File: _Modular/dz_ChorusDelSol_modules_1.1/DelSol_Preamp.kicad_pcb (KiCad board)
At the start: 2 copper layers, 110.5 x 38.1 mm, 79 parts, among them J1 Filter Switch, J2 BBD Drive, J3 Dry LMR In, J4 Eq Pot Hi, J5 Eq Pot Mid, J6 Eq Pot Low, J7 Power, U1 LM2904, U2 MCP601, U3 LM2902

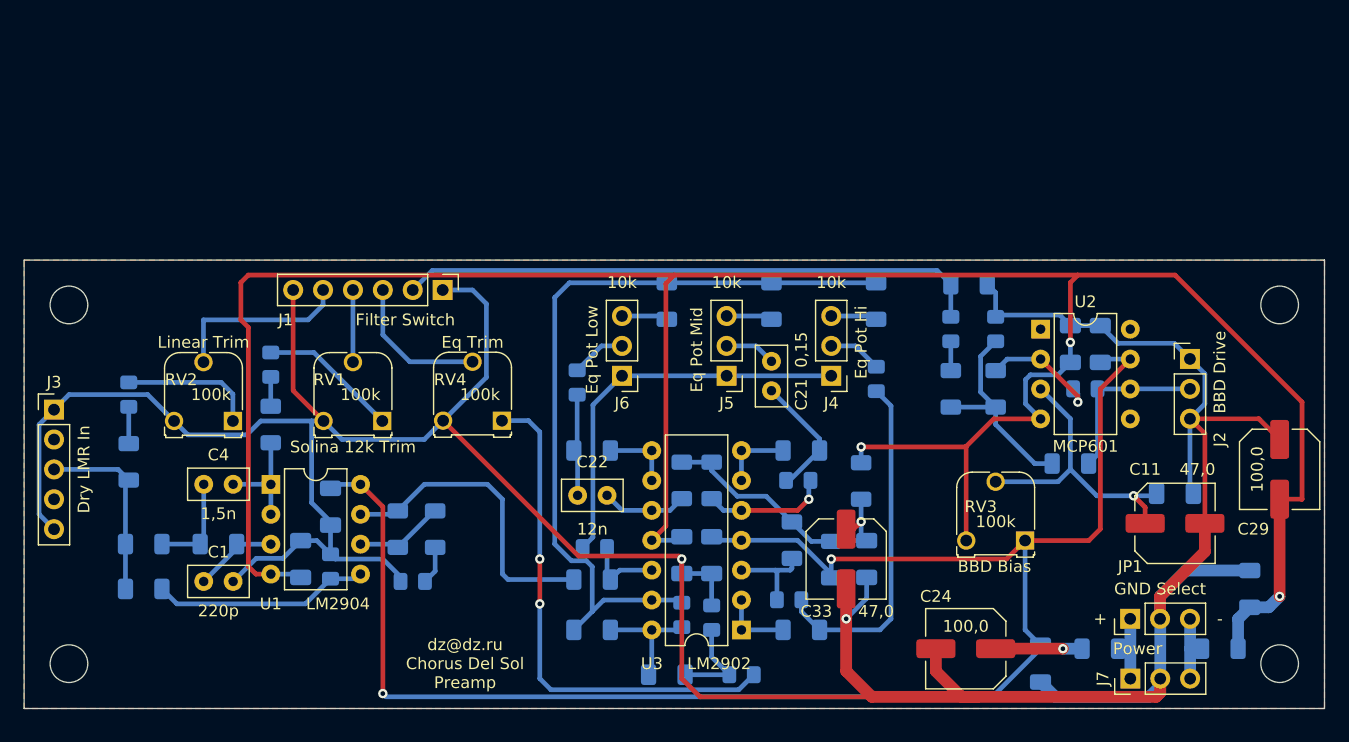
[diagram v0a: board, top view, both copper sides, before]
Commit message: up
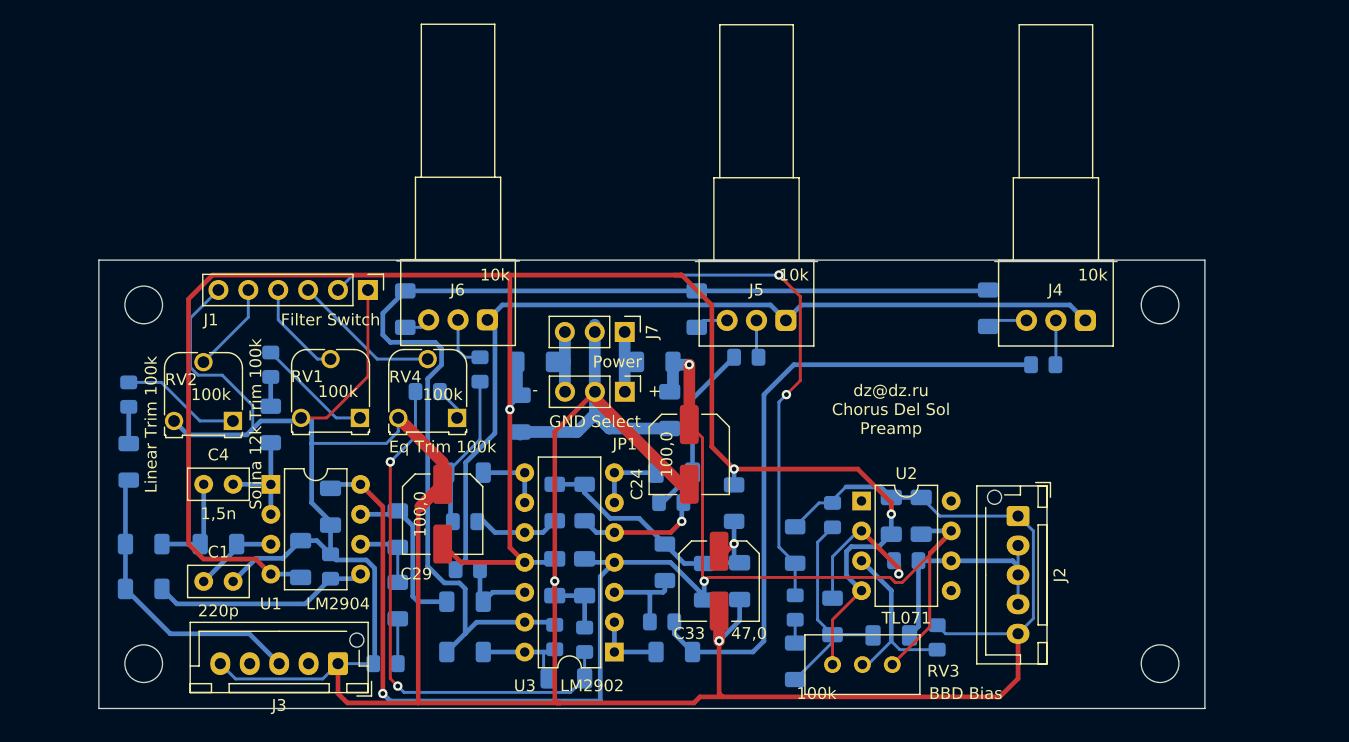
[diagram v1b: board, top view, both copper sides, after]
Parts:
- removed C12: 0,1, Capacitor_SMD:C_1206_3216Metric_Pad1.33x1.80mm_HandSolder
- C11: value 47,0 -> 10,0; footprint Capacitor_SMD:C_Elec_6.3x5.8 -> Capacitor_SMD:C_0805_2012Metric_Pad1.18x1.45mm_HandSolder; moved to B.Cu
- C21, C22: footprint Capacitor_THT:C_Disc_D5.0mm_W2.5mm_P2.50mm -> Capacitor_SMD:C_0805_2012Metric_Pad1.18x1.45mm_HandSolder; moved to B.Cu
- J2: footprint Connector_PinHeader_2.54mm:PinHeader_1x03_P2.54mm_Vertical -> Connector_JST:JST_XH_B5B-XH-AM_1x05_P2.50mm_Vertical
- J3: footprint Connector_PinHeader_2.54mm:PinHeader_1x05_P2.54mm_Vertical -> Connector_JST:JST_XH_B5B-XH-AM_1x05_P2.50mm_Vertical
- J4: value Eq Pot Hi -> Eq Pot 10k; footprint Connector_PinHeader_2.54mm:PinHeader_1x03_P2.54mm_Vertical -> Potentiometer_THT:Potentiometer_Alps_RK097_Single_Horizontal
- J5: value Eq Pot Mid -> Eq Pot 10k; footprint Connector_PinHeader_2.54mm:PinHeader_1x03_P2.54mm_Vertical -> Potentiometer_THT:Potentiometer_Alps_RK097_Single_Horizontal
- J6: value Eq Pot Low -> Eq Pot 10k; footprint Connector_PinHeader_2.54mm:PinHeader_1x03_P2.54mm_Vertical -> Potentiometer_THT:Potentiometer_Alps_RK097_Single_Horizontal
- RV1: value Solina 12k Trim -> Solina 12k Trim 100k
- RV2: value Linear Trim -> Linear Trim 100k
- RV3: footprint Potentiometer_THT:Potentiometer_Runtron_RM-065_Vertical -> Potentiometer_THT:Potentiometer_Bourns_3296W_Vertical
- RV4: value Eq Trim -> Eq Trim 100k
- U2: value MCP601 -> TL071
- moved C29 71.2 mm to (87.6, 39.4)
- moved C30 63.8 mm to (94.2, 30.8), turned to 90 degrees
- moved R26 63.1 mm to (95.5, 26.4), turned to 180 degrees
- moved J7 52.1 mm to (103.1, 23.9), turned to -90 degrees
- moved JP1 47.1 mm to (103.1, 29.0), turned to -90 degrees
- moved R24 45.0 mm to (105.7, 26.4), turned to 0 degrees
- moved C25 38.2 mm to (106.9, 30.5)
- moved C13 35.9 mm to (86.4, 28.9)
- moved J3 32.4 mm to (78.7, 52.1), turned to 180 degrees
- moved C24 28.7 mm to (108.6, 34.3), turned to -90 degrees
- moved C7 27.1 mm to (117.6, 47.3)
- moved R6 26.7 mm to (117.6, 51.9)
- moved R8 26.6 mm to (117.6, 42.0), turned to -90 degrees
- moved R7 23.8 mm to (120.8, 48.1)
- moved C11 22.4 mm to (129.7, 49.8), turned to 90 degrees
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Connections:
- J2 pad 3: GND -> Net-(C6-Pad1)
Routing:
- net /-V: track 216.9 -> 166.7 mm
- net Net-(C14-Pad1): track 33.8 -> 75.9 mm
- net Net-(C13-Pad1): track 43.7 -> 2.85 mm, vias 2 -> 0
- net Net-(C13-Pad2): track 8.19 -> 45.0 mm, vias 0 -> 2
- net Net-(C17-Pad1): track 66.9 -> 96.6 mm
- net /+V: track 153.5 -> 128.0 mm
- net Net-(C18-Pad2): track 29.5 -> 54.3 mm
- net Net-(C7-Pad1): track 49.7 -> 66.4 mm, vias 0 -> 2
- net GND: track 298.8 -> 312.3 mm
- net Net-(R10-Pad1): track 26.3 -> 14.2 mm
- net Net-(RV3-Pad2): track 25.9 -> 15.4 mm, vias 1 -> 0
- net /Dry Mix: track 16.1 -> 25.1 mm
- net Net-(J1-Pad5): track 15.5 -> 7.71 mm
- net Net-(C6-Pad1): track 14.5 -> 20.3 mm
- net Net-(C20-Pad2): track 10.7 -> 15.2 mm
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- removed copper zone on F.Cu, net GND
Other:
- board size 110.5 x 38.1 mm -> 94 x 38.1 mm
